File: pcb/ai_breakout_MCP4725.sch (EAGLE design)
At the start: 10 parts, among them J1 1X03, J2 1X03NOFIRST, U1 MCP4725

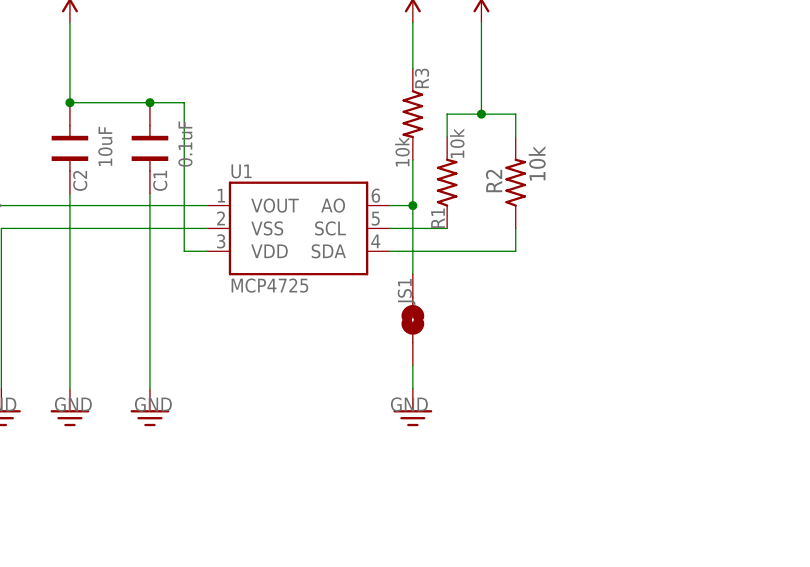
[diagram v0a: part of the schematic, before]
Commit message: gerber file created
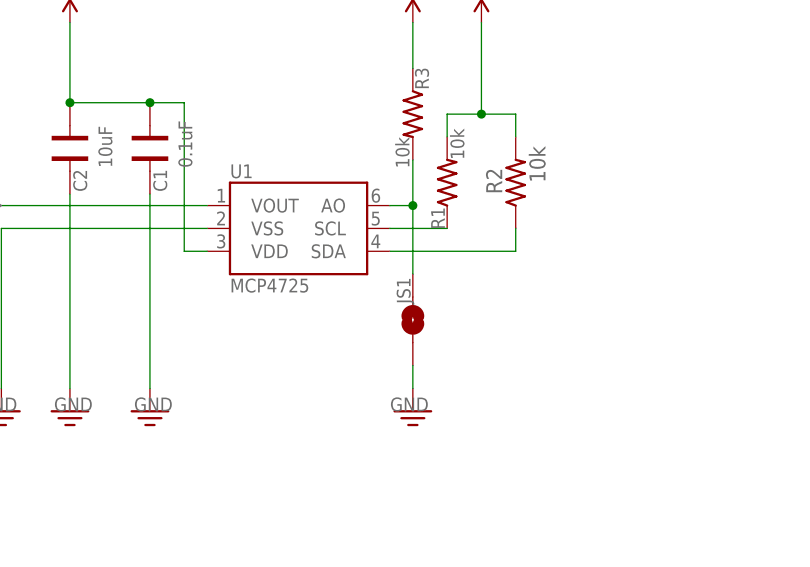
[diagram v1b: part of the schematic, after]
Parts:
- U1: value MCP4725 -> MCP4725SOT-23
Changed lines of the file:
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@@
 <part name="R3" library="Ai_Passives" deviceset="RES" device="0603" value="10k"/>
 <part name="FRAME1" library="frames" deviceset="A3L-LOC" device=""/>
-<part name="U1" library="Ai_IC" deviceset="MCP4725" device="SOT-23" value="MCP4725"/>
+<part name="U1" library="Ai_IC" deviceset="MCP4725" device="SOT-23" value="MCP4725SOT-23"/>
 <part name="J1" library="Ai_Connectors" deviceset="1X03" device=""/>
 <part name="J2" library="Ai_Connectors" deviceset="1X03" device="NOFIRST" value="1X03NOFIRST"/>
